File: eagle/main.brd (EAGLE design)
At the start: 73 x 41.3 mm, 25 parts, among them IC1 74LS595D, IC3 317EMP, IC4 74LS595D, Q1 BSS123, Q2 BSS123, Q3 BSS123, Q4 BSS123, Q5 BSS123

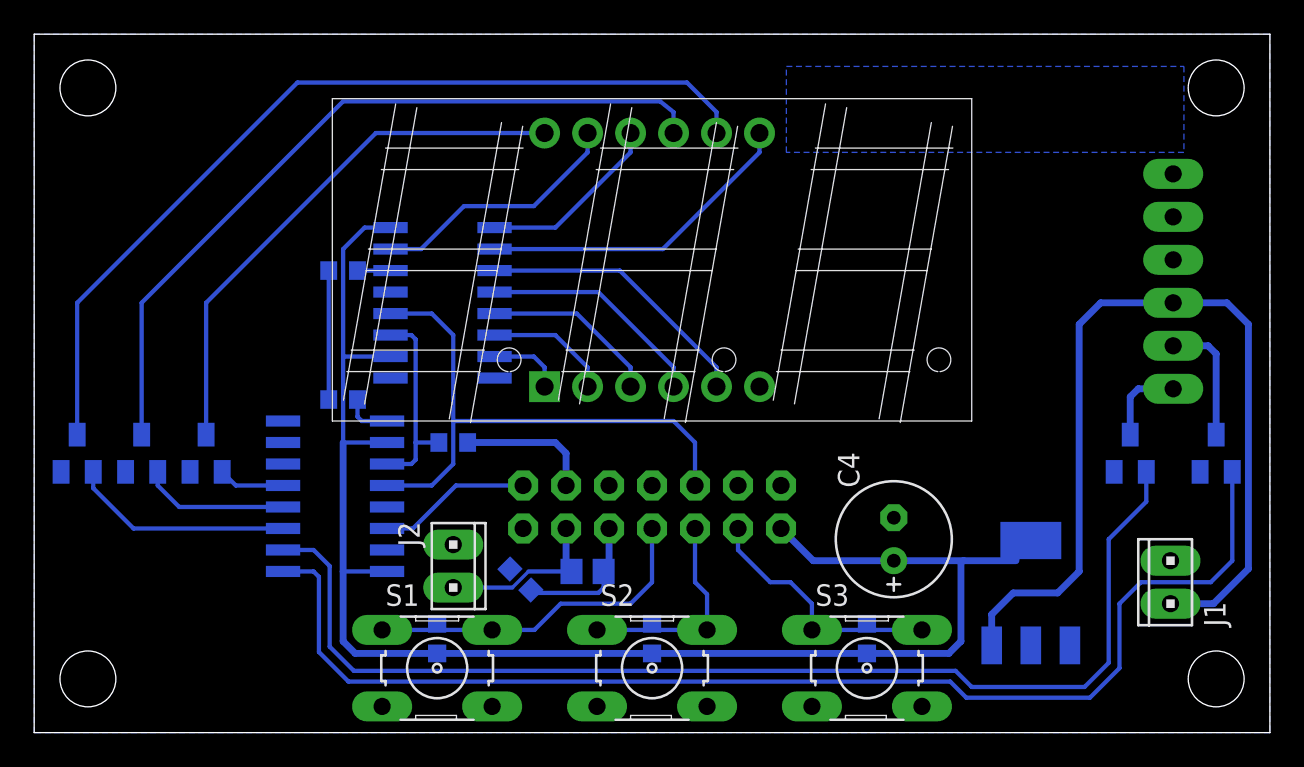
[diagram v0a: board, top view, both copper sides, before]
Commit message: Tidied up the swath of damage i put in last night.
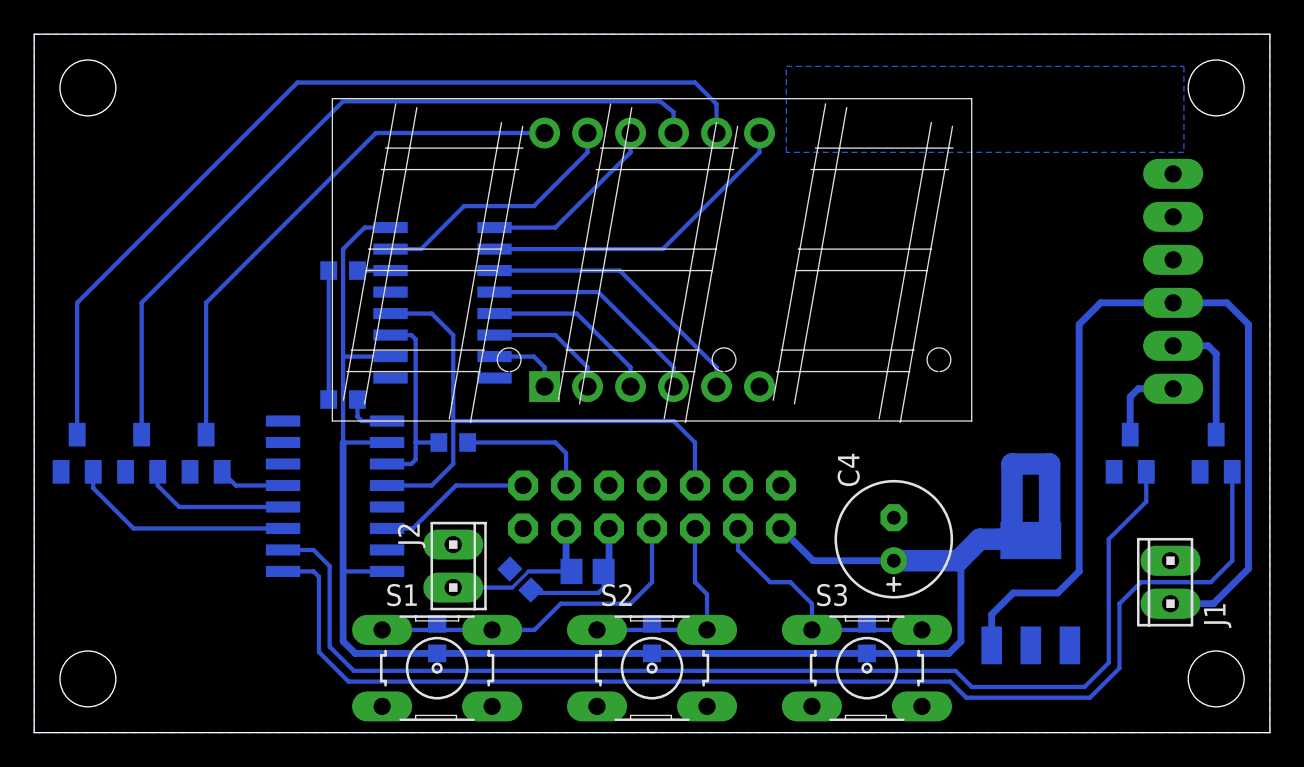
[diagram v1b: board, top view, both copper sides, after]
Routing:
- net VCC: track 92.6 -> 105.3 mm
- added copper zone on layer 16, net VCC
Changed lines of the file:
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@@
 <wire x1="2.54" y1="17.61" x2="2.54" y2="25.4" width="0.254" layer="16"/>
 <wire x1="2.54" y1="25.4" x2="15.5575" y2="38.4175" width="0.254" layer="16"/>
-<wire x1="15.5575" y1="38.4175" x2="38.57625" y2="38.4175" width="0.254" layer="16"/>
-<wire x1="38.57625" y1="38.4175" x2="40.3225" y2="36.67125" width="0.254" layer="16"/>
-<wire x1="40.3225" y1="36.67125" x2="40.3225" y2="35.433" width="0.254" layer="16"/>
+<wire x1="15.5575" y1="38.4175" x2="39.0525" y2="38.4175" width="0.254" layer="16"/>
+<wire x1="39.0525" y1="38.4175" x2="40.3225" y2="37.1475" width="0.254" layer="16"/>
+<wire x1="40.3225" y1="37.1475" x2="40.3225" y2="35.433" width="0.254" layer="16"/>
 </signal>
 <signal name="N$10">
@@
 <contactref element="IC3" pad="4"/>
 <contactref element="430" pad="1"/>
-<wire x1="58.01975" y1="10.16" x2="58.89625" y2="11.354" width="0.254" layer="16"/>
+<wire x1="58.33725" y1="11.43" x2="58.89625" y2="11.354" width="0.254" layer="16"/>
 <contactref element="C4" pad="+"/>
 <wire x1="44.1325" y1="12.065" x2="46.0375" y2="10.16" width="0.4064" layer="16"/>
 <wire x1="46.0375" y1="10.16" x2="50.8" y2="10.16" width="0.4064" layer="16"/>
-<wire x1="58.01975" y1="10.16" x2="54.9275" y2="10.16" width="0.4064" layer="16"/>
+<wire x1="58.33725" y1="11.43" x2="57.785" y2="11.43" width="1.27" layer="16"/>
+<wire x1="57.15" y1="11.43" x2="55.88" y2="11.43" width="1.27" layer="16"/>
+<wire x1="55.88" y1="11.43" x2="54.61" y2="10.16" width="1.27" layer="16"/>
 <contactref element="IC4" pad="10"/>
 <contactref element="IC1" pad="10"/>
@@
 <contactref element="C2" pad="2"/>
 <contactref element="C3" pad="2"/>
-<wire x1="54.9275" y1="10.16" x2="50.8" y2="10.16" width="0.4064" layer="16"/>
+<wire x1="54.61" y1="10.16" x2="50.8" y2="10.16" width="1.27" layer="16"/>
 <wire x1="23.8125" y1="4.68125" x2="36.5125" y2="4.68125" width="0.4064" layer="16"/>
 <wire x1="36.5125" y1="4.68125" x2="49.2125" y2="4.68125" width="0.4064" layer="16"/>
@@
 <wire x1="54.0525" y1="4.68125" x2="54.76875" y2="5.3975" width="0.4064" layer="16"/>
 <wire x1="54.76875" y1="5.3975" x2="54.76875" y2="10.00125" width="0.4064" layer="16"/>
-<wire x1="54.76875" y1="10.00125" x2="54.9275" y2="10.16" width="0.254" layer="16"/>
+<wire x1="54.76875" y1="10.00125" x2="54.61" y2="10.16" width="0.254" layer="16"/>
 <wire x1="18.25625" y1="17.145" x2="20.8534" y2="17.145" width="0.254" layer="16"/>
 <wire x1="21.0566" y1="22.225" x2="18.25625" y2="22.225" width="0.254" layer="16"/>
+<wire x1="57.785" y1="11.43" x2="57.785" y2="15.875" width="1.27" layer="16"/>
+<wire x1="57.785" y1="15.875" x2="60.0075" y2="15.875" width="1.27" layer="16"/>
+<wire x1="60.0075" y1="15.875" x2="60.0075" y2="11.43" width="1.27" layer="16"/>
+<wire x1="60.0075" y1="11.43" x2="58.33725" y2="11.43" width="1.27" layer="16"/>
+<wire x1="57.785" y1="11.43" x2="57.15" y2="11.43" width="1.27" layer="16"/>
+<polygon width="0.254" layer="16">
+<vertex x="57.785" y="15.875"/>
+<vertex x="57.785" y="11.43"/>
+<vertex x="60.0075" y="11.43"/>
+<vertex x="60.0075" y="15.875"/>
+<vertex x="57.94375" y="15.875"/>
+</polygon>
 </signal>
 <signal name="GND">
@@
 <contactref element="R4" pad="1"/>
 <contactref element="430" pad="12"/>
-<wire x1="25.615" y1="17.145" x2="30.7975" y2="17.145" width="0.4064" layer="16"/>
-<wire x1="30.7975" y1="17.145" x2="31.4325" y2="16.51" width="0.4064" layer="16"/>
-<wire x1="31.4325" y1="16.51" x2="31.4325" y2="14.605" width="0.4064" layer="16"/>
+<wire x1="25.615" y1="17.145" x2="30.7975" y2="17.145" width="0.254" layer="16"/>
+<wire x1="30.7975" y1="17.145" x2="31.4325" y2="16.51" width="0.254" layer="16"/>
+<wire x1="31.4325" y1="16.51" x2="31.4325" y2="14.605" width="0.254" layer="16"/>
 </signal>
 <signal name="N$30">
